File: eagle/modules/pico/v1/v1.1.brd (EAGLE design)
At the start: 93.3 x 53.3 mm, 41 parts, among them IC1 MEGA8-AI, IC3 ULN2803A, IC4 ULN2803A, J1 RJ12STRAIGHT-RS232-SERVER

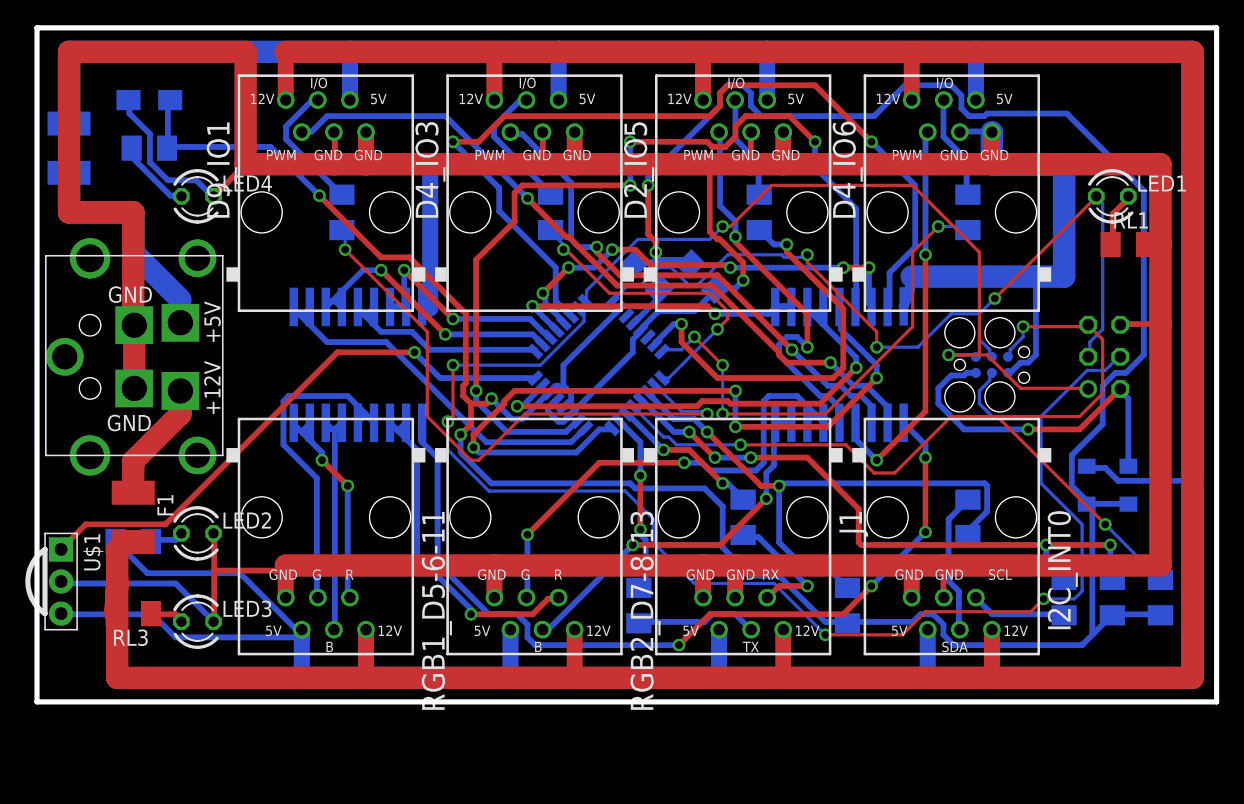
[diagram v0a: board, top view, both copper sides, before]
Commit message: Update pico
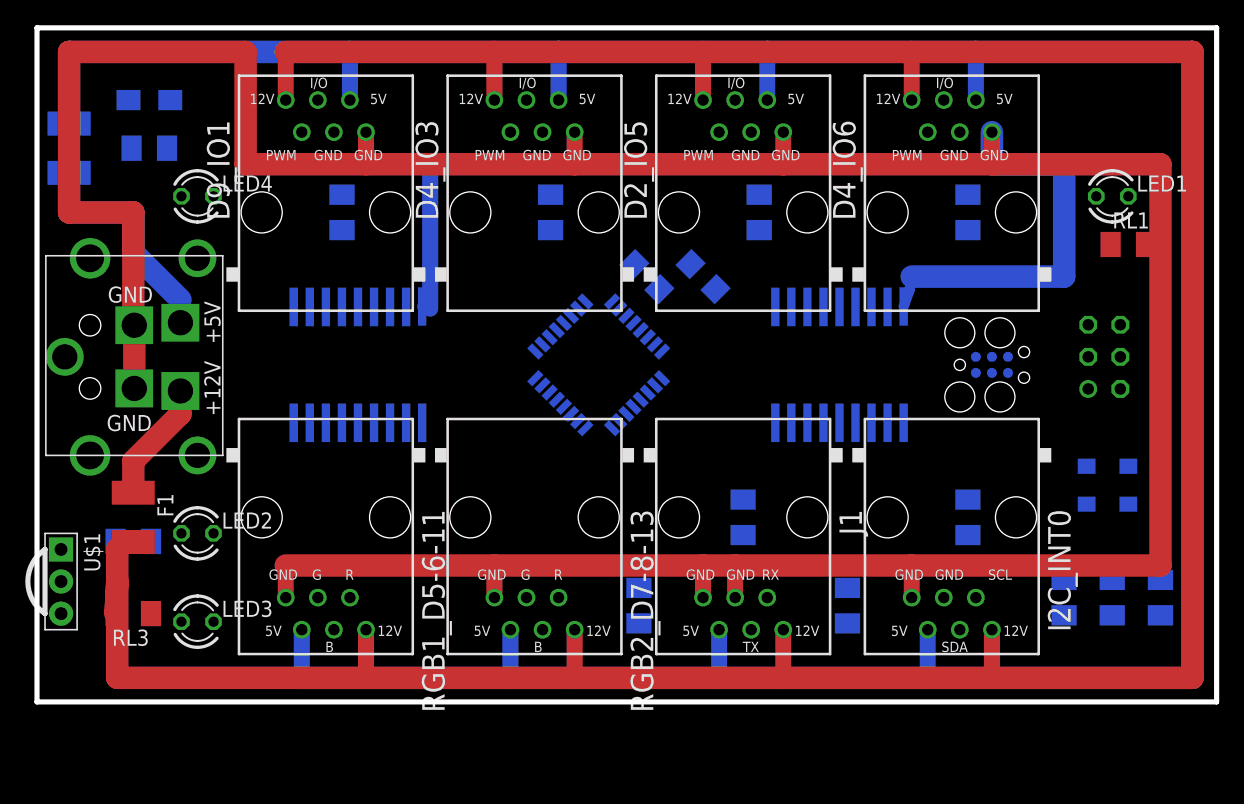
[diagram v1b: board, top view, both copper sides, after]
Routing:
- net 5V: track 233.2 -> 0.00 mm, vias 5 -> 0
- net MOSI: track 110.3 -> 0.00 mm, vias 4 -> 0
- net GND: track 403.2 -> 301.8 mm, vias 1 -> 0
- net RESET: track 74.2 -> 0.00 mm, vias 3 -> 0
- net D4: track 71.6 -> 0.00 mm, vias 4 -> 0
- net D10: track 70.5 -> 0.00 mm, vias 2 -> 0
- net SCK: track 67.5 -> 0.00 mm, vias 3 -> 0
- net COM: track 66.6 -> 0.00 mm, vias 4 -> 0
- net MISO: track 60.2 -> 0.00 mm, vias 2 -> 0
- net N$51: track 57.8 -> 0.00 mm, vias 2 -> 0
- net D2: track 57.7 -> 0.00 mm, vias 4 -> 0
- net SCL: track 49.7 -> 0.00 mm, vias 5 -> 0
- net A3: track 47.7 -> 0.00 mm, vias 2 -> 0
- net +5V: track 291.4 -> 245.1 mm
- net SDA: track 46.2 -> 0.00 mm, vias 2 -> 0
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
